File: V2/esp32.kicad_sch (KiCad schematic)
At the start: 5 parts, among them J11 RJ45_LED, U11 PCF8574, U12 LAN8710A, U13 ESP32-WROOM-32, U14 CH340T

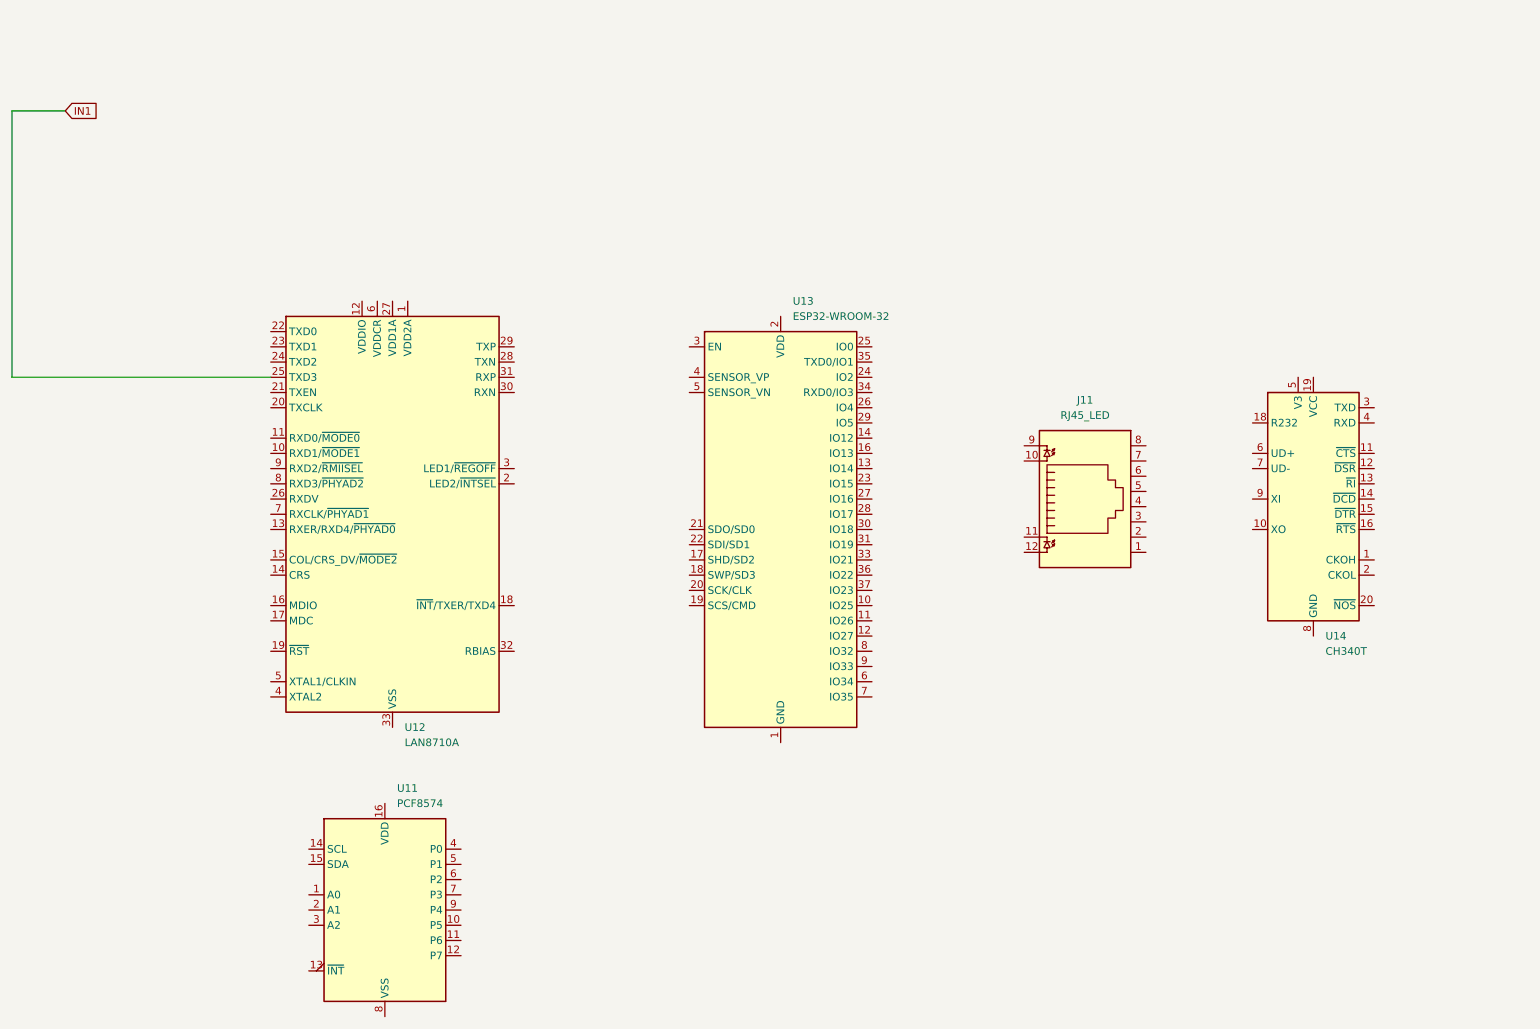
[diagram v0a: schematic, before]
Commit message: Development
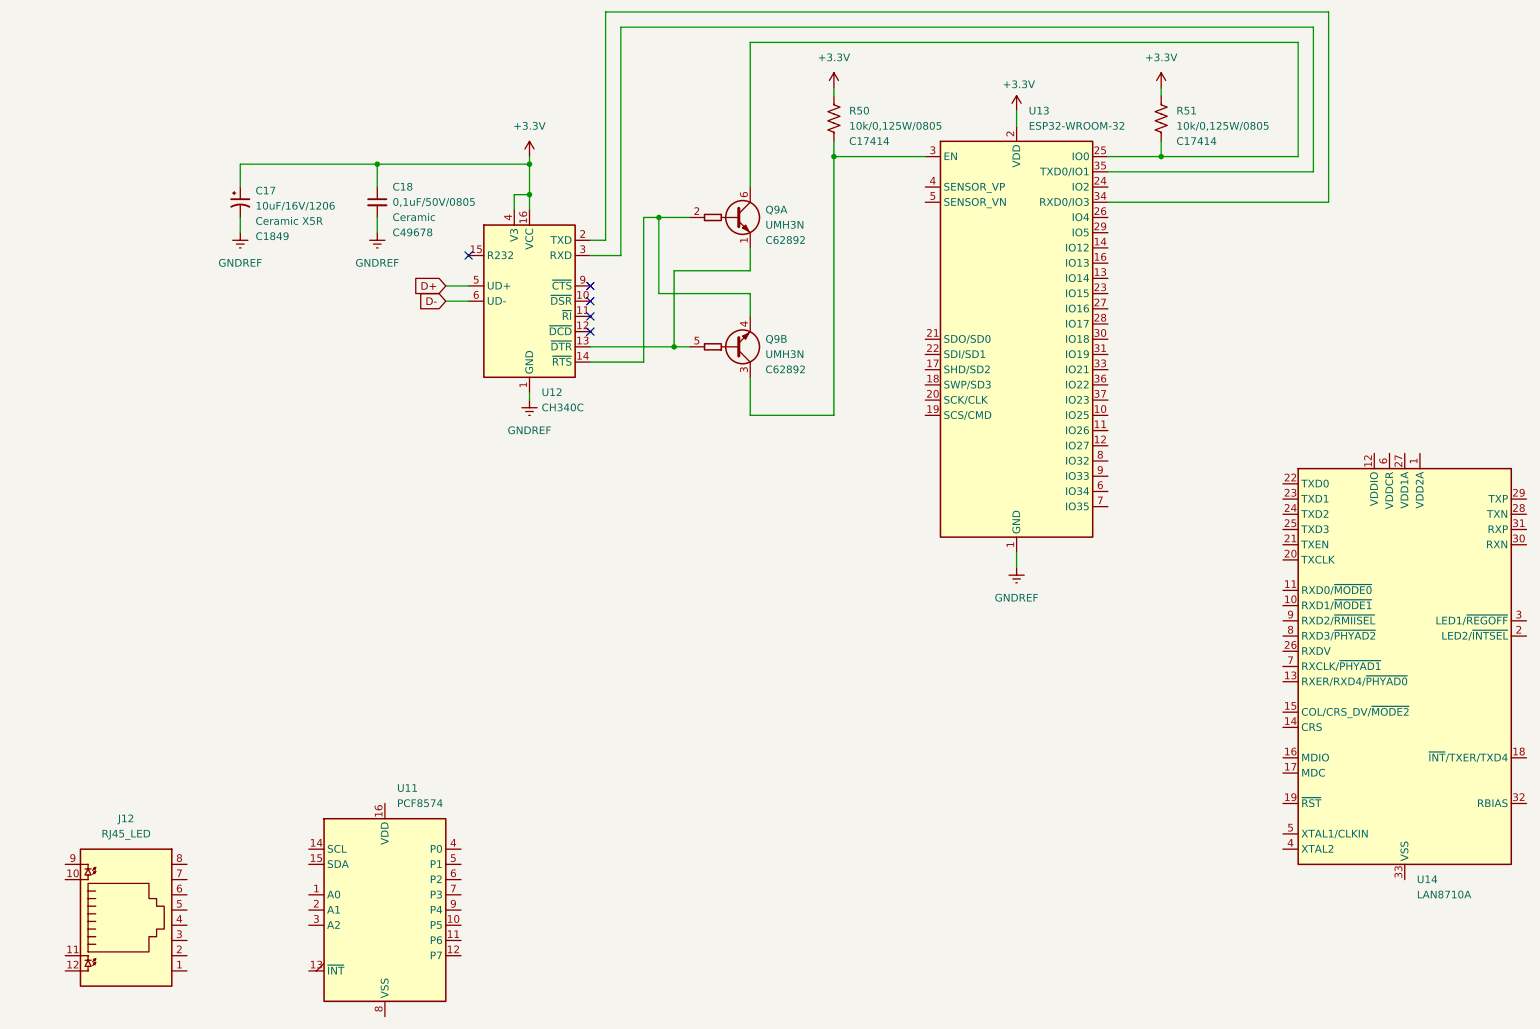
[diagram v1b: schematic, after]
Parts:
- removed U14: CH340T, Package_SO:SSOP-20_5.3x7.2mm_P0.65mm, symbol Interface_USB:CH340T
- added C17: 10uF/16V/1206, Tales:C_1206_3216Metric, symbol Device:C_Polarized_Small_US
- added C18: 0,1uF/50V/0805, Tales:C_0805_2012Metric, symbol Device:C_Small
- added Q9: UMH3N, Package_TO_SOT_SMD:SOT-363_SC-70-6, symbol Transistor_BJT:UMH3N
- added R50, R51: 10k/0,125W/0805, Tales:R_0805_2012Metric, symbol Device:R_US
- added U12: CH340C, Package_SO:SOIC-16_3.9x9.9mm_P1.27mm, symbol Interface_USB:CH340C
- renumbered J11 to J12, U12 to U14
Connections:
- net GNDREF: now reaches U13.1 (GND), U13.15 (GND), U13.38 (GND), U13.39 (GND)
- net GNDREF: now also C17.2, C18.2, U12.1 (GND)
- net +3.3V: now reaches U13.2 (VDD)
- net +3.3V: now also C17.1, C18.1, R50.1, R51.1, U12.16 (VCC), U12.4 (V3)
- net at U13.25 (IO0): now also Q9.6 (C1), R51.2
- net at U13.3 (EN): now also Q9.3 (C2), R50.2
- net at U13.34 (RXD0/IO3): now also U12.2 (TXD)
- net at U13.35 (TXD0/IO1): now also U12.3 (RXD)
- net IN1: no longer names the net of U14.25 (TXD3)
- new net: Q9.1 (E1), Q9.5 (B2), U12.13 (~{DTR})
- new net: Q9.2 (B1), Q9.4 (E2), U12.14 (~{RTS})
- new net D+: U12.5 (UD+)
- new net D-: U12.6 (UD-)
- no-connect marks 0 -> 5
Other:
- moved on the sheet: J12, U13, U14
